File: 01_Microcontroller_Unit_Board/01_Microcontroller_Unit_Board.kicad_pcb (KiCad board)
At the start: 4 copper layers, 25.7 x 68 mm, 36 parts, among them J1 10118192-0001LF, J2 TSM-103-01-S-SV, J3 61301811121, J4 61301811121, Q1 BC847BDW1T1G, SW1 B3U-1000P, SW2 B3U-1000P

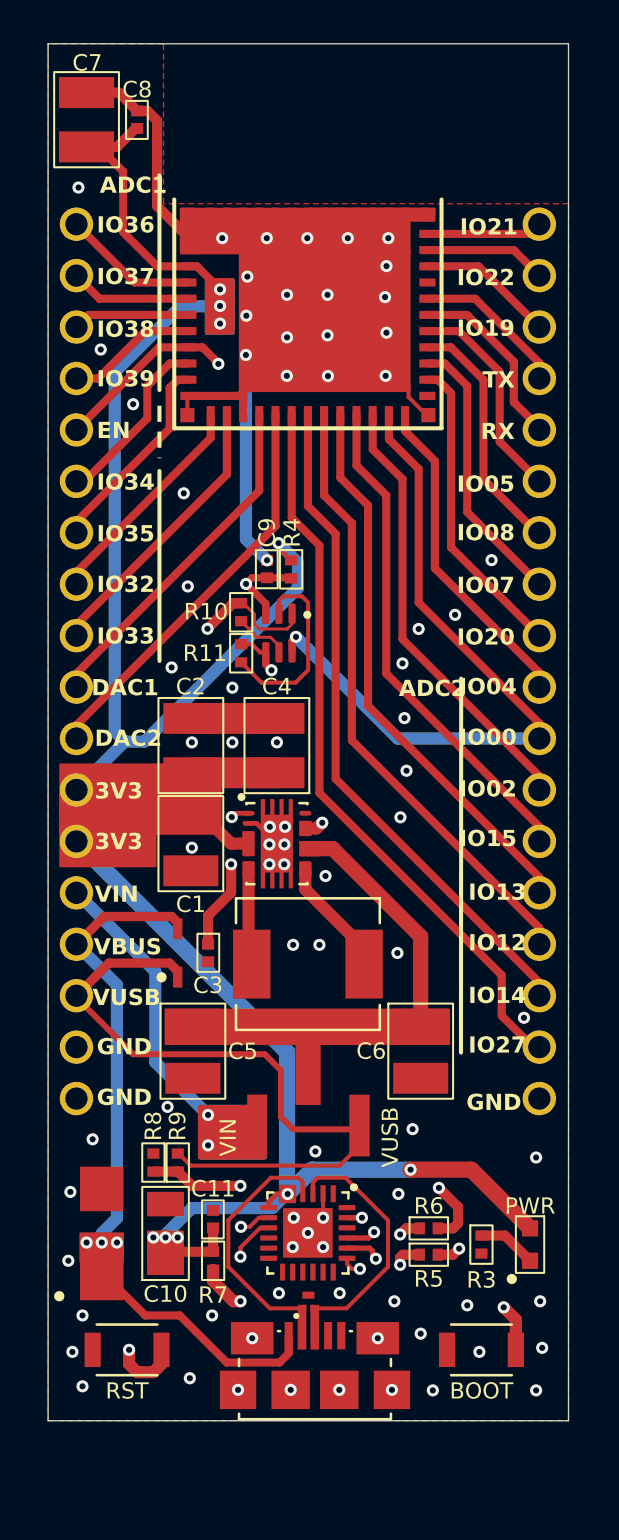
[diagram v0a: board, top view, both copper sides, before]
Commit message: Final check on PCBs, completed on Aug 25, 2026
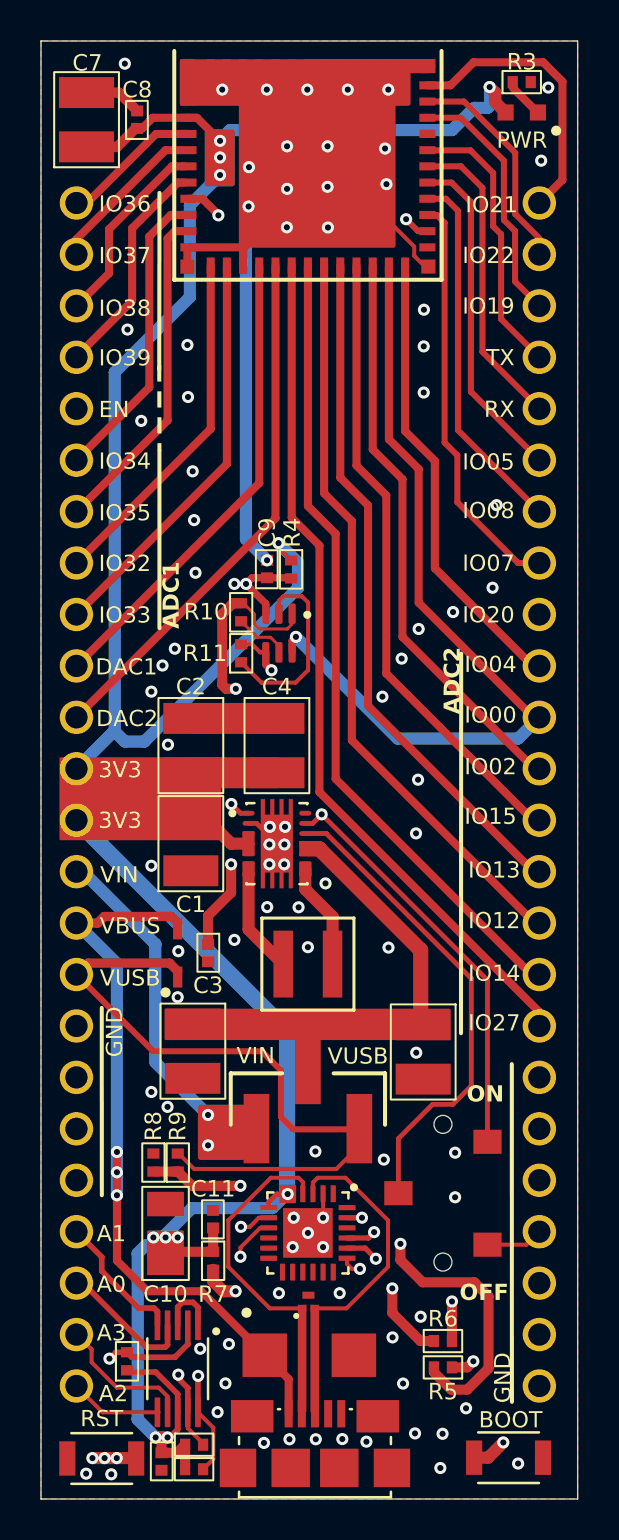
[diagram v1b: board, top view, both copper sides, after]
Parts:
- added C12: 0.1µF(±10%), Capacitors:0402 (1005 Metric), F.Cu at (144.2, 131.2)
- added DAIC1: ADS1115IDGSR, Data Acquisition ICs:10-VSSOP, F.Cu at (145.0, 126.6)
- added R12: 10kΩ(±1%), Resistors:0402 (1005 Metric), F.Cu at (142.5, 126.2)
- added R13: 10kΩ(±1%), Resistors:0402 (1005 Metric), F.Cu at (145.8, 131.5)
- added R14: 10kΩ(±1%), Resistors:0402 (1005 Metric), F.Cu at (145.8, 130.3)
- added SW3: CL-SB-12B-01T, Switches:Nidec_CL-SB-12B-01T, F.Cu at (158.1, 117.9)
- J3, J4: value 61301811121 -> 61302411121; footprint Connector Assemblies:Wurth_61301811121 -> Connector Assemblies:Wurth_61302411121
- L1: footprint Inductors:TDK_SPM6530T-1R5M-HZ -> Inductors:Coilcraft_XFL4020-152MEC
- moved R3 57.4 mm to (162.0, 63.0), turned to 0 degrees
- moved D4 55.9 mm to (162.0, 64.5), turned to 180 degrees
- moved D3 11.9 mm to (151.5, 125.9), turned to 0 degrees
- moved MCU1 7.34 mm to (151.4, 64.5)
- moved J3 6.57 mm to (140.0, 98.2)
- moved J4 6.57 mm to (162.9, 98.2)
- moved R6 5.61 mm to (158.1, 125.2)
- moved R5 5.61 mm to (158.1, 126.5)
- moved SW1 5.51 mm to (141.2, 131.0)
- moved SW2 5.49 mm to (161.3, 131.0), turned to 0 degrees
- moved J1 3.85 mm to (151.8, 128.8)
- moved G*** 0.52 mm to (159.4, 88.5)
- moved C6 0.13 mm to (157.1, 110.9)
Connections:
- C3 pad 1: Net-(PMIC1-EN) -> Net-(PMIC1-PS/SYNC)
- PMIC1 pad 1: Net-(PMIC1-EN) -> Net-(PMIC1-PS/SYNC)
- PMIC1 pad 13: Net-(PMIC1-EN) -> Net-(PMIC1-PS/SYNC)
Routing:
- net GPIO21: track 5.73 -> 90.3 mm, vias 0 -> 1
- net GPIO22: track 6.05 -> 86.3 mm, vias 0 -> 1
- net GPIO35/ADC1_CH7: track 10.2 -> 64.8 mm, vias 0 -> 1
- net Net-(PMIC1-PS/SYNC): track 0.00 -> 33.8 mm, vias 0 -> 3
- net EN: track 69.0 -> 102.4 mm, vias 3 -> 6
- net +3V3: track 114.4 -> 141.4 mm, vias 9 -> 11
- net GPIO0/ADC2_CH1: track 65.2 -> 79.3 mm
- net RXD0: track 52.4 -> 64.9 mm
- net TXD0: track 52.9 -> 65.2 mm
- net GPIO20: track 15.2 -> 25.5 mm, vias 0 -> 1
- net Net-(PMIC1-EN): track 14.4 -> 23.8 mm, vias 3 -> 0
- net Net-(CIIC1-TXD): track 8.23 -> 16.2 mm
- net AIN3: track 0.00 -> 6.86 mm
- net AIN0: track 0.00 -> 6.82 mm
- net AIN1: track 0.00 -> 6.72 mm
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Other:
- board size 25.7 x 68 mm -> 26.5 x 72 mm
- board text added: "A0"
- board text added: "A1"
- board text added: "A2"
- board text added: "A3"
- board text added: "OFF"
- board text added: "ON"
